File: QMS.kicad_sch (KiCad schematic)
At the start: 12 parts, among them J1 Screw_Terminal_01x02, J2 PINHD_1x5_Male, J3 PINHD_1x3_Male, U1 ESP-12E, U2 AMS1117-3.3

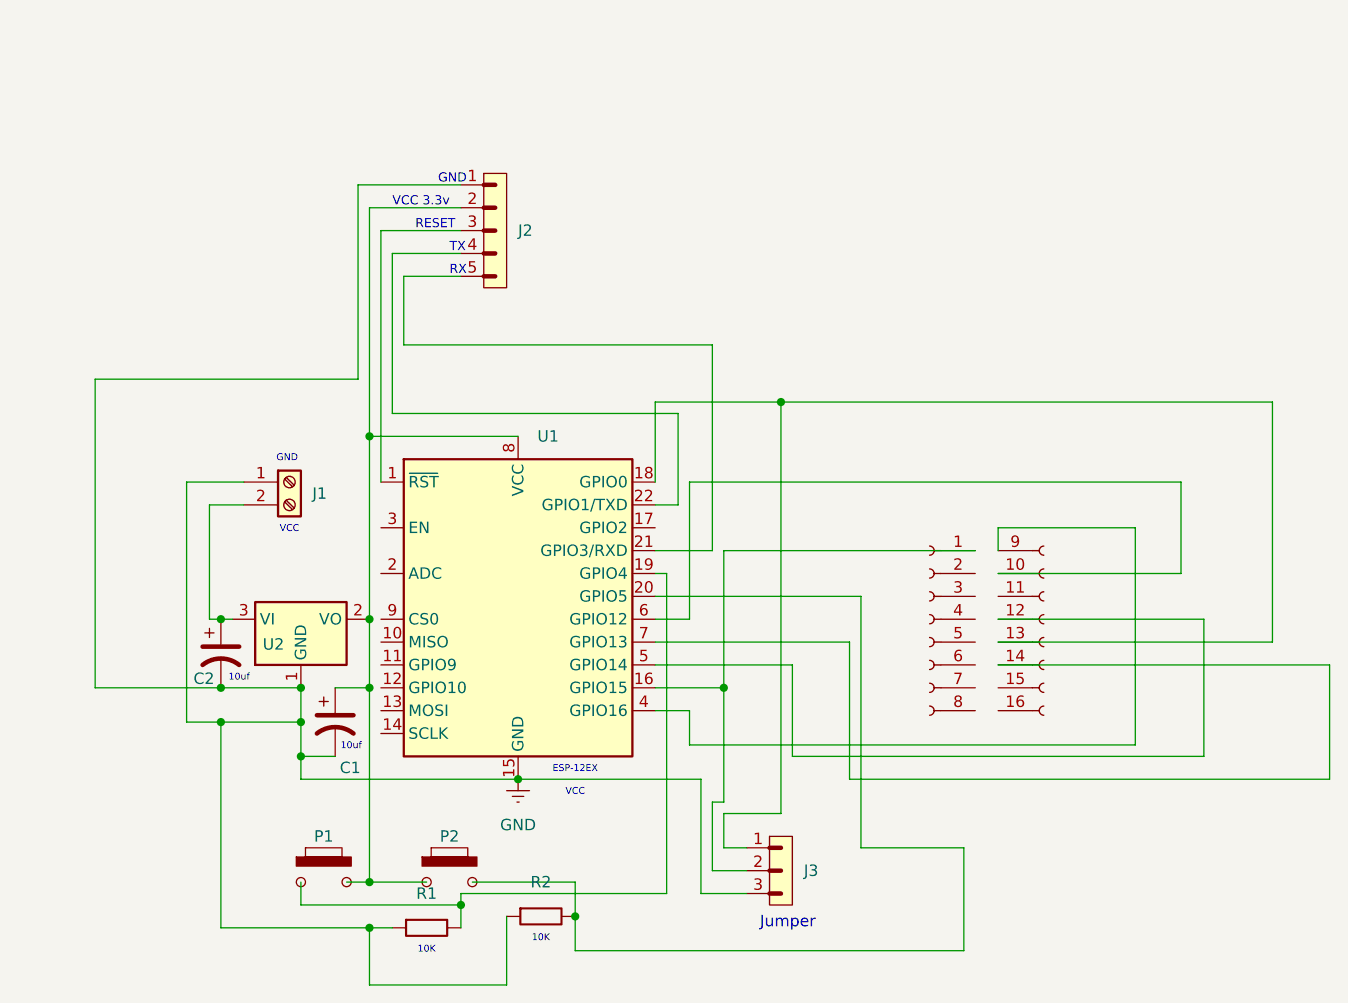
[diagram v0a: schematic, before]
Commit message: updated accordin to suggested rules
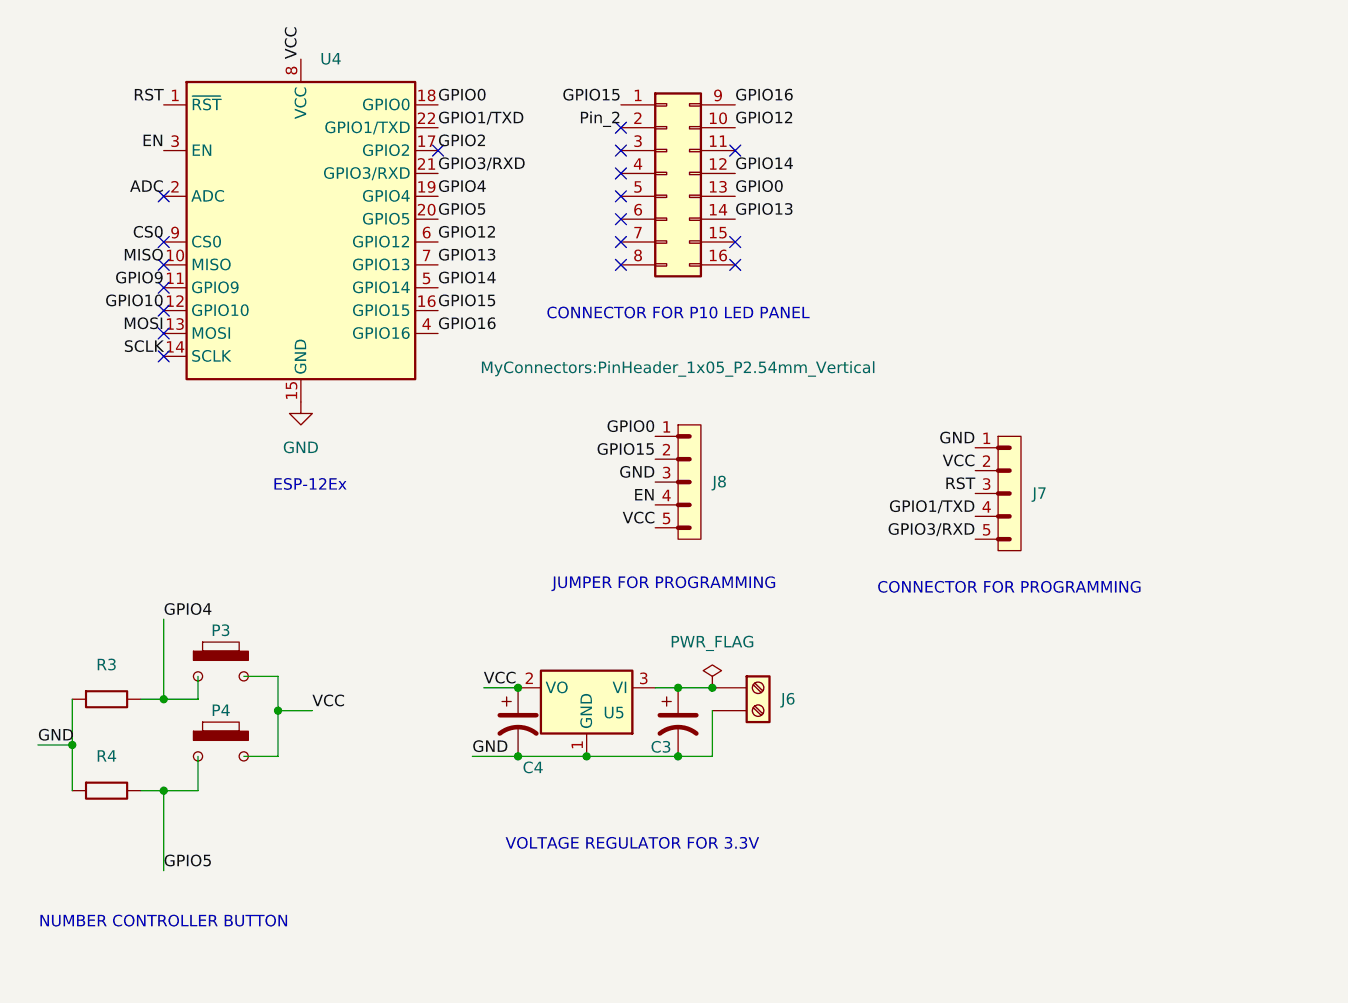
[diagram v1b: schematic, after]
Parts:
- removed C1, C2: C_Polarized_US, Capacitor_THT:CP_Radial_D6.3mm_P2.50mm, symbol Device:C_Polarized_US
- removed J1: Screw_Terminal_01x02, TerminalBlock:TerminalBlock_MaiXu_MX126-5.0-02P_1x02_P5.00mm, symbol Connector:Screw_Terminal_01x02
- removed J2: PINHD_1x5_Male, Connector_PinHeader_2.54mm:PinHeader_1x05_P2.54mm_Vertical, symbol PCM_SL_Pin_Headers:PINHD_1x5_Male
- removed J3: PINHD_1x3_Male, Connector_PinHeader_2.54mm:PinHeader_1x03_P2.54mm_Vertical, symbol PCM_SL_Pin_Headers:PINHD_1x3_Male
- removed P1, P2: ~, Button_Switch_THT:SW_PUSH-12mm, symbol PCM_Nuova-Elettronica-Switches:Push_Button
- removed R1, R2: Resistor, Resistor_THT:R_Axial_DIN0207_L6.3mm_D2.5mm_P7.62mm_Horizontal, symbol PCM_SL_Resistors:Resistor
- removed U1: ESP-12E, RF_Module:ESP-12E, symbol RF_Module:ESP-12E
- removed U2: AMS1117-3.3, Package_TO_SOT_SMD:SOT-223-3_TabPin2, symbol Regulator_Linear:AMS1117-3.3
- removed U3: ~, MyConnectors:Hub16, symbol New_Library:HUB16
- added C3, C4: C_Polarized_US, MyConnectors:CP_Radial_D6.3mm_P2.50mm, symbol Device:C_Polarized_US
- added J4: Conn_02x08_Top_Bottom, MyConnectors:PinHeader 2x8 p2.54mm, symbol Connector_Generic:Conn_02x08_Top_Bottom
- added J6: Screw_Terminal_01x02, TerminalBlock:TerminalBlock_MaiXu_MX126-5.0-02P_1x02_P5.00mm, symbol Connector:Screw_Terminal_01x02
- added J7, J8: PINHD_1x5_Male, MyConnectors:PinHeader_1x05_P2.54mm_Vertical, symbol PCM_SL_Pin_Headers:PINHD_1x5_Male
- added P3, P4: ~, MyConnectors:PUSH_BTN_12x12mm, symbol PCM_Nuova-Elettronica-Switches:Push_Button
- added R3, R4: Resistor, MyConnectors:R_Axial_DIN0207_L6.3mm_D2.5mm_P7.62mm_Horizontal, symbol PCM_SL_Resistors:Resistor
- added U4: ESP-12E, RF_Module:ESP-12E, symbol RF_Module:ESP-12E
- added U5: AMS1117-3.3, Package_TO_SOT_SMD:SOT-223-3_TabPin2, symbol Regulator_Linear:AMS1117-3.3
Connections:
- net GND: now also C3.2, C4.2, J6.2 (Pin_2), J7.1, J8.3, R3.1, R4.1, U4.15 (GND), U5.1 (GND)
- new net: C3.1, J6.1 (Pin_1), U5.3 (VI)
- new net ADC: U4.2 (ADC)
- new net CS0: U4.9 (CS0)
- new net EN: J8.4, U4.3 (EN)
- new net GPIO0: J4.13 (Pin_13), J8.1, U4.18 (GPIO0)
- new net GPIO1/TXD: U4.22 (GPIO1/TXD)
- new net GPIO10: U4.12 (GPIO10)
- new net GPIO12: J4.10 (Pin_10), U4.6 (GPIO12)
- new net GPIO13: J4.14 (Pin_14), U4.7 (GPIO13)
- new net GPIO14: J4.12 (Pin_12), U4.5 (GPIO14)
- new net GPIO15: J4.1 (Pin_1), J8.2, U4.16 (GPIO15)
- new net GPIO16: J4.9 (Pin_9), U4.4 (GPIO16)
- new net GPIO1/TXD: J7.4
- new net GPIO2: U4.17 (GPIO2)
- new net GPIO3/RXD: U4.21 (GPIO3/RXD)
- new net GPIO3/RXD: J7.5
- new net GPIO4: P3.1, R3.2, U4.19 (GPIO4)
- new net GPIO5: P4.1, R4.2, U4.20 (GPIO5)
- new net GPIO9: U4.11 (GPIO9)
- new net MISO: U4.10 (MISO)
- new net MOSI: U4.13 (MOSI)
- new net Pin_2: J4.2 (Pin_2)
- new net RST: J7.3, U4.1 (~{RST})
- new net SCLK: U4.14 (SCLK)
- new net VCC: C4.1, J7.2, J8.5, P3.2, P4.2, U4.8 (VCC), U5.2 (VO)
- no-connect marks 0 -> 18
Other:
- note added: "CONNECTOR FOR P10 LED PANEL"
- note added: "CONNECTOR FOR PROGRAMMING"
- note added: "ESP-12Ex"
- note added: "JUMPER FOR PROGRAMMING"
- note added: "NUMBER CONTROLLER BUTTON"
- note added: "VOLTAGE REGULATOR FOR 3.3V"
- note removed: "10K"
- note removed: "10uf"
- note removed: "ESP-12EX"
- note removed: "GND"
- note removed: "Jumper"
- note removed: "RESET"
- note removed: "RX"
- note removed: "TX"
- note removed: "VCC"
- note removed: "VCC 3.3v"
